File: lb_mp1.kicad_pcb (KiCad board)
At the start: 2 copper layers, 100 x 100 mm, 156 parts, among them J1 USB_POWER, J2 USB_HOST, J3 AudioJack4_SwitchTR1, J4 RJ45_LED_Shielded, J5 Micro_SD_Card, J7 SERIAL, J8 UART_Header, J9 Bat, SW1 SW_SPDT, SW2 SW_SPDT, U1 V3S-split, U10 FPC_40, U11 STM32F030C8Tx, U2 SRV05-4, U3 SY8088AAC, U4 W25Q128JVS, U5 FEMDRM008G-58A39_NO_NC, U6 AMS1117-3.3, U7 CH340N, U8 AXP209, U9 SY7200AABC, Y1 32.768khz, Y2 24MHz

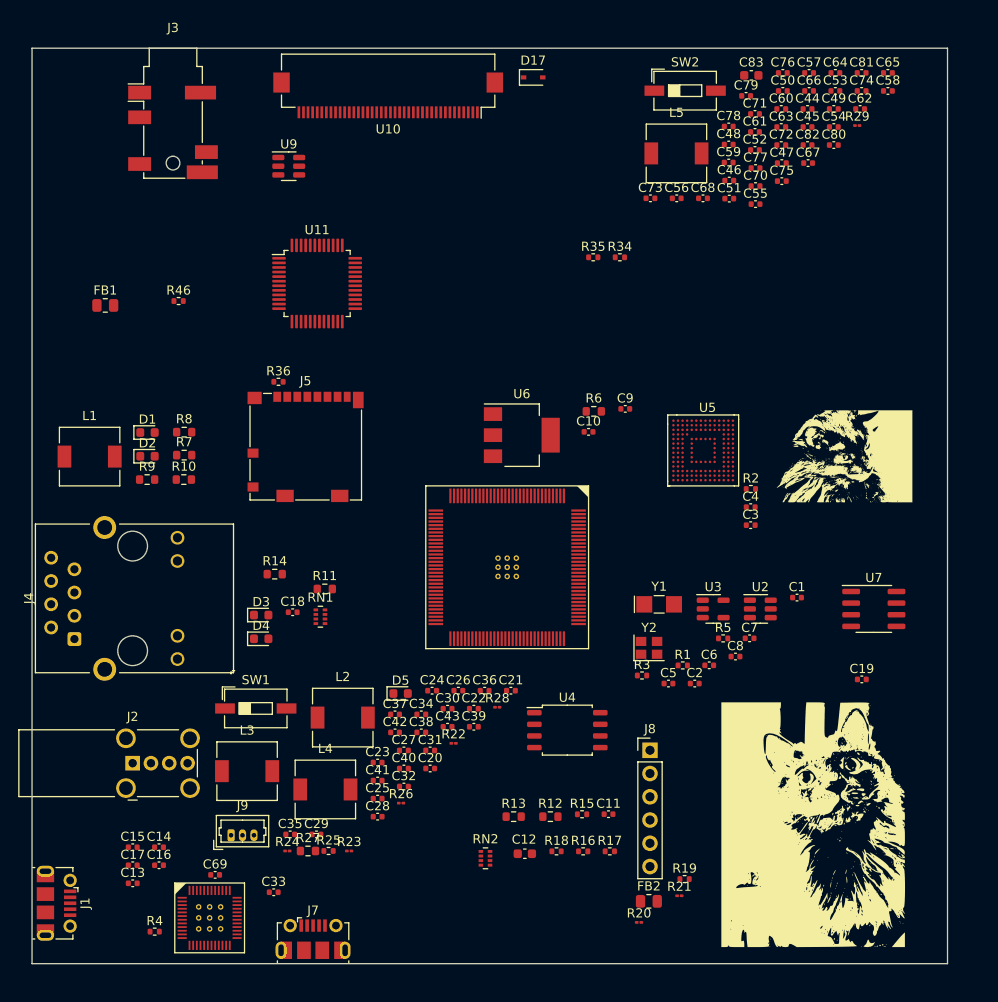
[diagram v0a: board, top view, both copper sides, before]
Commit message: cleaning and naming
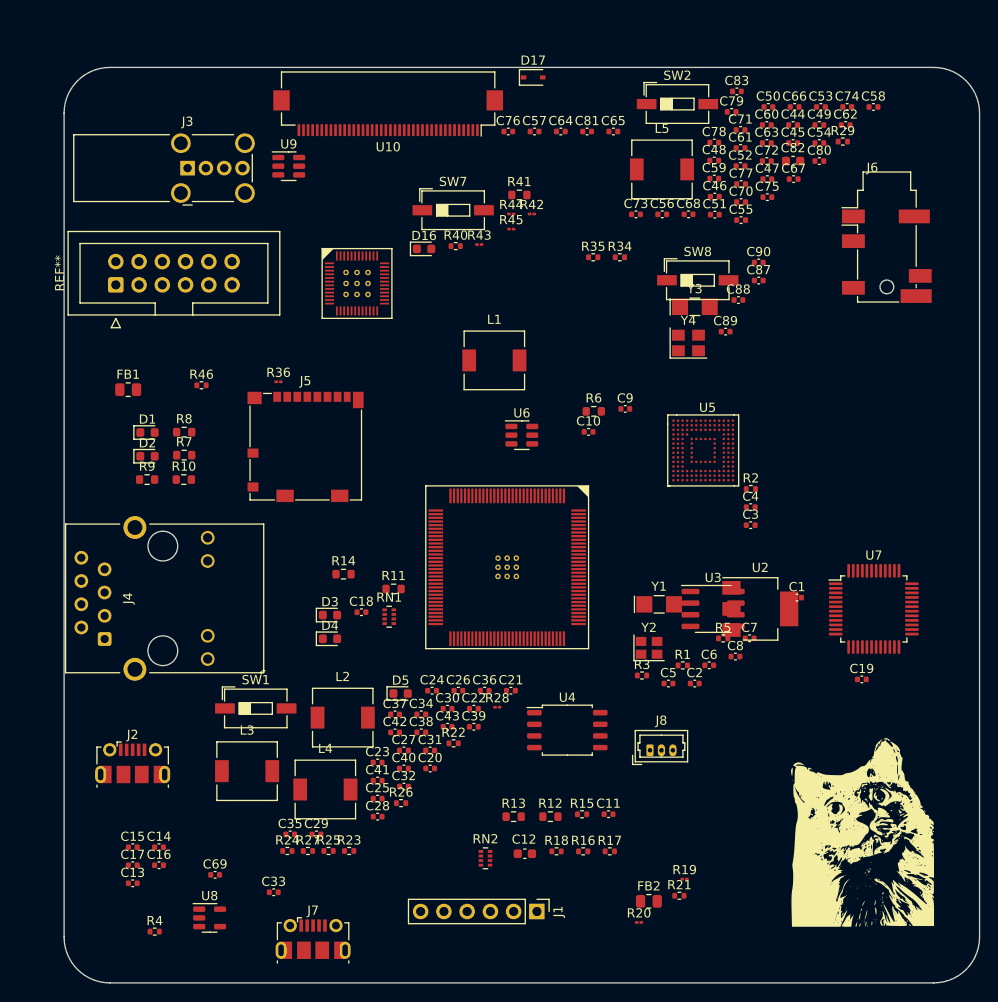
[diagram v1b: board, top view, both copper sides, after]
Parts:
- removed the G*** at (175.2, 72.5)
- removed the G*** at (171.8, 112.7)
- removed J9: Bat, Connector_Molex:Molex_PicoBlade_53047-0310_1x03_P1.25mm_Vertical
- added C87: 12pf, Capacitor_SMD:C_0402_1005Metric, F.Cu at (165.9, 53.3)
- added C88: 12pf, Capacitor_SMD:C_0402_1005Metric, F.Cu at (163.7, 55.4)
- added C89: 18pf, Capacitor_SMD:C_0402_1005Metric, F.Cu at (162.3, 58.9)
- added C90: 18pf, Capacitor_SMD:C_0402_1005Metric, F.Cu at (165.9, 51.3)
- added D16: LED, LED_SMD:LED_0603_1608Metric, F.Cu at (129.3, 49.8)
- added G***: LOGO, LOGO, F.Cu at (175.0, 116.1)
- added J6: AudioJack4_SwitchTR1, Connector_Audio:Jack_3.5mm_PJ31060-I_Horizontal, F.Cu at (179.9, 50.6)
- added R40: 0R, Resistor_SMD:R_0402_1005Metric, F.Cu at (132.8, 49.5)
- added R41: 0.03R, Resistor_SMD:R_0603_1608Metric, F.Cu at (139.7, 43.9)
- added R42: 1k, Resistor_SMD:R_01005_0402Metric, F.Cu at (141.1, 46.0)
- added R43: 200k 1%, Resistor_SMD:R_01005_0402Metric, F.Cu at (135.4, 49.4)
- added R44: 47k, Resistor_SMD:R_01005_0402Metric, F.Cu at (138.8, 46.0)
- added R45: 10k, Resistor_SMD:R_01005_0402Metric, F.Cu at (138.8, 47.7)
- added REF**: IDC-Header_2x06_P2.54mm_Vertical, Connector_IDC:IDC-Header_2x06_P2.54mm_Vertical, F.Cu at (95.7, 53.8)
- added SW7: SW_SPDT, Button_Switch_SMD:SW_DIP_SPSTx01_Slide_6.7x4.1mm_W6.73mm_P2.54mm_LowProfile_JPin, F.Cu at (132.5, 45.6)
- added SW8: SW_SPDT, Button_Switch_SMD:SW_DIP_SPSTx01_Slide_6.7x4.1mm_W6.73mm_P2.54mm_LowProfile_JPin, F.Cu at (159.2, 53.2)
- added Y3: 32.768khz, Crystal:Crystal_SMD_MicroCrystal_CC7V-T1A-2Pin_3.2x1.5mm_HandSoldering, F.Cu at (158.9, 56.1)
- added Y4: 16MHz, Crystal:Crystal_SMD_3225-4Pin_3.2x2.5mm, F.Cu at (158.2, 60.1)
- C11, C19, C67: value 100n -> 10u
- C18: value 0.1uF -> 10u
- C2: value 10u -> 0.1uF
- C22, C27, C41, C42: value 10uF -> 100n
- C23, C25: value 1nF -> 1u
- C24, C26, C39: value 10uF -> 1u
- C28: value 100n -> 1u
- C29, C36: value 1uF -> 100n
- C30: value 4.7uF -> 1u
- C31, C32: value 4.7uF -> 100n
- C33: value 1uF -> 10n
- C34: value 100uF -> 100n
- C35: value 4.7u -> 100n
- C37, C43: value 0.22uF -> 100n
- C38, C44, C46, C48, C50: value 1u -> 100n
- C40: value 10uF -> 10u
- C45: value 1u -> 10u
- C5, C6: value 10u -> 100n
- C52, C56, C61, C63, C65, C66: value 100n -> 10uF
- C54, C60: value 100n -> 4.7uF
- C57, C68, C78: value 100n -> 1uF
- C58: value 1u -> 4.7uF
- C59: value 10u -> 4.7uF
- C62, C64: value 100n -> 1nF
- C69: value 4.7uF -> 100uF
- C70: value 100pF -> 4.7u
- C71: value 10n -> 100pF
- C72: value 10u -> 1uF
- C73: value 100n -> 0.22uF
- C74: value 100pF -> 10uF
- C75: value 10u -> 10uF
- C77: value 100n -> 100pF
- C80: value 1uF -> 4.7uF
- C81: value 4.7uF -> 10uF
- C82: footprint Capacitor_SMD:C_0402_1005Metric -> Capacitor_SMD:C_0603_1608Metric
- C83: value 10uF -> 0.22uF; footprint Capacitor_SMD:C_0603_1608Metric -> Capacitor_SMD:C_0402_1005Metric
- J1: value USB_POWER -> UART_Header; footprint Connector_USB:USB_Micro-B_Molex-105017-0001 -> Connector_PinHeader_2.54mm:PinHeader_1x06_P2.54mm_Vertical
- J2: value USB_HOST -> SERIAL; footprint Connector_USB:USB_A_Wuerth_614004134726_Horizontal -> Connector_USB:USB_Micro-B_Molex-105017-0001
- J3: value AudioJack4_SwitchTR1 -> USB_HOST; footprint Connector_Audio:Jack_3.5mm_PJ31060-I_Horizontal -> Connector_USB:USB_A_Wuerth_614004134726_Horizontal
- J7: value SERIAL -> USB_POWER
- J8: value UART_Header -> Bat; footprint Connector_PinHeader_2.54mm:PinHeader_1x06_P2.54mm_Vertical -> Connector_Molex:Molex_PicoBlade_53047-0310_1x03_P1.25mm_Vertical
- R19: value 47k -> 470; footprint Resistor_SMD:R_0402_1005Metric -> Resistor_SMD:R_01005_0402Metric
- R21: value 470 -> 47k; footprint Resistor_SMD:R_01005_0402Metric -> Resistor_SMD:R_0402_1005Metric
- R22: value 2.2R -> 33R; footprint Resistor_SMD:R_01005_0402Metric -> Resistor_SMD:R_0402_1005Metric
- R23: value 1k -> 10k; footprint Resistor_SMD:R_01005_0402Metric -> Resistor_SMD:R_0402_1005Metric
- R24: value 47k -> 33R; footprint Resistor_SMD:R_01005_0402Metric -> Resistor_SMD:R_0402_1005Metric
- R25: value 47k -> 33R
- R26: value 200k 1% -> 0R; footprint Resistor_SMD:R_01005_0402Metric -> Resistor_SMD:R_0402_1005Metric
- R27: value 0.03R -> 22R; footprint Resistor_SMD:R_0603_1608Metric -> Resistor_SMD:R_0402_1005Metric
- R29: value 1k -> 47k; footprint Resistor_SMD:R_01005_0402Metric -> Resistor_SMD:R_0402_1005Metric
- R36: value 33R -> 1k; footprint Resistor_SMD:R_0402_1005Metric -> Resistor_SMD:R_01005_0402Metric
- R46: value 0R -> 10k
- U11: value STM32F030C8Tx -> AXP209; footprint Package_QFP:LQFP-48_7x7mm_P0.5mm -> Allwinner:AXP209-QFN48
- U2: value SRV05-4 -> AMS1117-3.3; footprint Package_TO_SOT_SMD:SOT-23-6 -> Package_TO_SOT_SMD:SOT-223-3_TabPin2
- U3: value SY8088AAC -> CH340N; footprint Package_TO_SOT_SMD:SOT-23-5 -> Package_SO:SOIC-8_3.9x4.9mm_P1.27mm
- U6: value AMS1117-3.3 -> SRV05-4; footprint Package_TO_SOT_SMD:SOT-223-3_TabPin2 -> Package_TO_SOT_SMD:SOT-23-6
- U7: value CH340N -> STM32F030C8Tx; footprint Package_SO:SOIC-8_3.9x4.9mm_P1.27mm -> Package_QFP:LQFP-48_7x7mm_P0.5mm
- U8: value AXP209 -> SY8088AAC; footprint Allwinner:AXP209-QFN48 -> Package_TO_SOT_SMD:SOT-23-5
- moved J1 52.5 mm to (141.7, 122.2)
- moved L1 45.4 mm to (137.0, 62.0)
- moved C57 30.7 mm to (141.4, 37.0)
- moved C64 30.7 mm to (144.3, 37.0)
- moved C65 30.7 mm to (150.0, 37.0)
- moved C81 30.7 mm to (147.1, 37.0)
- moved C76 30.7 mm to (138.5, 37.0)
- moved FB1 9.53 mm to (97.0, 65.2)
- moved R46 9.53 mm to (105.0, 64.7)
- moved C18 7.51 mm to (122.5, 89.5)
- moved D3 7.51 mm to (119.0, 89.8)
- moved D4 7.51 mm to (119.0, 92.4)
- moved R11 7.51 mm to (126.0, 87.0)
- moved RN1 7.51 mm to (125.5, 90.0)
- moved R14 7.51 mm to (120.5, 85.3)
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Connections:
- C1 pad 2: Net-(C1-Pad2) -> GND
- C11 pad 1: +3.3V -> +1V2
- C18 pad 1: Net-(C18-Pad1) -> +1V2
- C19 pad 1: Net-(C19-Pad1) -> +3.3V
- C2 pad 1: +1V2 -> Net-(C2-Pad1)
- C22 pad 1: +1V2 -> +3.3V
- C24 pad 1: +3.3V -> +1V2
- C26 pad 1: +3.3V -> +1V8
- C29 pad 1: GND -> +1V2
- C29 pad 2: VDD -> GND
- C30 pad 1: GND -> +1V2
- C30 pad 2: +3V0 -> GND
- C31 pad 1: GND -> +3.3V
- C31 pad 2: Net-(C31-Pad2) -> GND
- C32 pad 1: Net-(C32-Pad1) -> +1V8
- C33 pad 1: GND -> +VDC
- C33 pad 2: Net-(C33-Pad2) -> GND
- C34 pad 1: GND -> VDD
- C34 pad 2: Net-(C34-Pad2) -> GND
- C35 pad 1: GND -> +3V0
- C35 pad 2: Net-(C35-Pad2) -> GND
- C36 pad 1: Net-(C36-Pad1) -> +1V2
- C37 pad 1: VCC -> +1V2
- C38 pad 1: +1V2 -> +3.3V
- C39 pad 1: VCC -> +1V8
- C40 pad 1: VCC -> +3V0
- C41 pad 1: VCC -> +1V2
- C42 pad 1: Net-(C42-Pad1) -> +1V2
- C43 pad 1: VCC -> +1V8
- C44 pad 1: +1V2 -> +3.3V
- C45 pad 1: +3.3V -> +VDC
- C46 pad 1: +1V8 -> +1V2
- C47 pad 1: +3.3V -> +1V2
- C48 pad 1: +3.3V -> +3V0
- C49 pad 1: +1V2 -> +VDC
- C5 pad 1: +1V2 -> +3.3V
- C50 pad 1: +1V2 -> +1V8
- C50 pad 2: GND -> Net-(C50-Pad2)
- C51 pad 1: +3.3V -> Net-(C50-Pad2)
- C52 pad 1: +1V8 -> VCC
- C53 pad 1: VDD -> +1V8
- C53 pad 2: GND -> Net-(C53-Pad2)
- C54 pad 1: +3V0 -> GND
- C54 pad 2: GND -> Net-(C54-Pad2)
- C55 pad 1: +1V2 -> +1V8
- C56 pad 1: +1V2 -> +1V8
- C57 pad 1: +3.3V -> GND
- C57 pad 2: GND -> VDD
- C58 pad 1: +1V8 -> GND
- C58 pad 2: GND -> +3V0
- C59 pad 1: +3V0 -> GND
- C59 pad 2: GND -> Net-(C59-Pad2)
- C6 pad 1: +3.3V -> Net-(C6-Pad1)
- C6 pad 2: GND -> Net-(C6-Pad2)
- C60 pad 1: +1V2 -> Net-(C60-Pad1)
- C62 pad 1: +1V8 -> +1V2
- C64 pad 1: +1V2 -> +3.3V
- C65 pad 1: +1V2 -> +3.3V
- C66 pad 1: +3V0 -> +3.3V
- C67 pad 1: +1V8 -> GND
- C67 pad 2: Net-(C67-Pad2) -> +VDC
- C68 pad 1: Net-(C67-Pad2) -> GND
- C68 pad 2: GND -> Net-(C68-Pad2)
- C70 pad 2: N_Oe -> Net-(C70-Pad2)
- C71 pad 1: +VDC -> GND
- C71 pad 2: GND -> N_Oe
- C72 pad 1: +VDC -> Net-(C72-Pad1)
- C73 pad 1: +VDC -> VCC
- C74 pad 1: GND -> VCC
- C74 pad 2: Pwron -> GND
- C75 pad 1: GND -> VCC
- C75 pad 2: +VDC -> GND
- C77 pad 1: +1V8 -> GND
- C77 pad 2: Net-(C77-Pad2) -> Pwron
- C78 pad 1: +1V8 -> +BATT
- C78 pad 2: GND -> Net-(C78-Pad2)
- C79 pad 1: +1V8 -> Net-(C78-Pad2)
- C80 pad 1: +BATT -> Net-(C80-Pad1)
- C80 pad 2: Net-(C42-Pad1) -> GND
- C81 pad 1: Net-(C81-Pad1) -> +BATT
- C82 pad 1: +BATT -> VCC
- FB1 pad 1: Net-(U11-Pad9) -> Net-(FB1-Pad1)
- FB1 pad 2: +3.3V -> Net-(C2-Pad1)
- FB2 pad 2: Net-(C18-Pad1) -> +3.3V
- J1 pad 1: +VDC -> GND
- J1 pad 4: Net-(J1-Pad4) -> Net-(D4-Pad1)
- J1 pad 5: GND -> Net-(D5-Pad1)
- J1 pad 6: GND -> unconnected-(J1-Pad6)
- J2 pad 1: VCC -> Net-(FB1-Pad1)
- J2 pad 4: GND -> Net-(J2-Pad4)
- J5 pad 1: Net-(D11-Pad1) -> Net-(D7-Pad1)
- J5 pad 2: Net-(D12-Pad1) -> Net-(D8-Pad1)
- J5 pad 5: Net-(D10-Pad1) (its old number) -> Net-(D6-Pad1)
- J5 pad 8: Net-(D15-Pad1) -> Net-(D11-Pad1)
- J7 pad 1: Net-(FB2-Pad1) -> +VDC
- J7 pad 2: Net-(J7-Pad2) -> unconnected-(J7-Pad2)
- J7 pad 3: Net-(J7-Pad3) -> unconnected-(J7-Pad3)
- J8 pad 1: GND -> +BATT
- J8 pad 2: unconnected-(J8-Pad2) -> GND
- J8 pad 3: unconnected-(J8-Pad3) -> (no net)
- L2 pad 1: +1V2 -> Net-(L2-Pad1)
- L2 pad 2: Net-(L2-Pad2) -> +1V8
- L3 pad 1: +3.3V -> +1V2
- L4 pad 1: Net-(L4-Pad1) -> +3.3V
- L4 pad 2: Net-(C42-Pad1) -> Net-(L4-Pad2)
- L5 pad 2: +1V8 -> Net-(C78-Pad2)
- R19 pad 1: Net-(J7-Pad4) -> +3.3V
- R19 pad 2: GND -> Net-(D4-Pad2)
- R20 pad 2: Net-(D3-Pad2) -> Net-(D5-Pad2)
- R21 pad 1: +3.3V -> Net-(J2-Pad4)
- R21 pad 2: Net-(D4-Pad2) -> GND
- R22 pad 1: +5V -> Net-(D6-Pad1)
- R22 pad 2: Net-(C20-Pad1) -> Net-(R22-Pad2)
- R23 pad 1: GND -> +3.3V
- R23 pad 2: N_Oe -> Net-(D7-Pad1)
- R24 pad 1: reset -> Net-(D14-Pad1)
- R24 pad 2: VDD -> Net-(R24-Pad2)
- R25 pad 1: Net-(J1-Pad4) -> Net-(D13-Pad1)
- R25 pad 2: GND -> Net-(R25-Pad2)
- R26 pad 1: GND -> Net-(C6-Pad2)
- R27 pad 1: Net-(C42-Pad1) -> GND
- R27 pad 2: +BATT -> Net-(C6-Pad1)
- R29 pad 1: Net-(R29-Pad1) -> Net-(J7-Pad4)
- R29 pad 2: Pwron -> GND
- R36 pad 1: Net-(D10-Pad1) (its old number) -> GND
- R36 pad 2: Net-(R36-Pad2) -> N_Oe
- R46 pad 1: VCC -> +3.3V
- R46 pad 2: Net-(C81-Pad1) -> Net-(U4-Pad3)
- RN1 pad 2: Net-(D12-Pad1) -> Net-(D8-Pad1)
- RN1 pad 5: Net-(D15-Pad1) -> Net-(D11-Pad1)
- U1 pad 101: Net-(D11-Pad1) -> Net-(D7-Pad1)
- U1 pad 102: Net-(D12-Pad1) -> Net-(D8-Pad1)
- U1 pad 105: Net-(R36-Pad2) -> Net-(R22-Pad2)
- U1 pad 107: Net-(D15-Pad1) -> Net-(D11-Pad1)
- U1 pad 110: Net-(J2-Pad2) -> Net-(J3-Pad2)
- U1 pad 111: Net-(J2-Pad3) -> Net-(J3-Pad3)
- U1 pad 120: Net-(R34-Pad2) -> Net-(R25-Pad2)
- U1 pad 121: Net-(R35-Pad2) -> Net-(R24-Pad2)
- U1 pad 124: Net-(C1-Pad2) -> Net-(C6-Pad2)
- U1 pad 125: Net-(R1-Pad2) -> Net-(R26-Pad2)
- U1 pad 48: Net-(D3-Pad1) -> Net-(D5-Pad1)
- U1 pad 63: Net-(C67-Pad2) -> Net-(C50-Pad2)
- U1 pad 71: Net-(C67-Pad2) -> Net-(C50-Pad2)
- U1 pad 73: Net-(R22-Pad2) -> Net-(R35-Pad2)
- U1 pad 97: Net-(C69-Pad2) -> Net-(C54-Pad2)
- U11 pad 1: +3.3V -> sda
- U11 pad 10: unconnected-(U11-Pad10) -> +1V2
- U11 pad 11: unconnected-(U11-Pad11) -> Net-(C60-Pad1)
- U11 pad 12: USART1_TX -> +3V0
- U11 pad 13: USART1_RX -> +3.3V
- U11 pad 14: unconnected-(U11-Pad14) -> VCC
- U11 pad 15: unconnected-(U11-Pad15) -> Net-(L4-Pad2)
- U11 pad 16: unconnected-(U11-Pad16) -> GND
- U11 pad 17: unconnected-(U11-Pad17) -> +3.3V
- U11 pad 19: unconnected-(U11-Pad19) -> Net-(C70-Pad2)
- U11 pad 2: unconnected-(U11-Pad2) -> scl
- U11 pad 21: unconnected-(U11-Pad21) -> VCC
- U11 pad 22: unconnected-(U11-Pad22) -> GND
- U11 pad 23: GND -> Net-(R43-Pad2)
- U11 pad 24: +3.3V -> Net-(C68-Pad2)
- U11 pad 25: unconnected-(U11-Pad25) -> reset
- U11 pad 26: unconnected-(U11-Pad26) -> Net-(C72-Pad1)
- U11 pad 27: unconnected-(U11-Pad27) -> Net-(C72-Pad1)
- U11 pad 28: unconnected-(U11-Pad28) -> VDD
- U11 pad 29: unconnected-(U11-Pad29) -> VCC
- U11 pad 30: unconnected-(U11-Pad30) -> Net-(C69-Pad2)
- U11 pad 31: unconnected-(U11-Pad31) -> Net-(C80-Pad1)
- U11 pad 32: unconnected-(U11-Pad32) -> +VDC
- U11 pad 33: unconnected-(U11-Pad33) -> +VDC
- U11 pad 34: unconnected-(U11-Pad34) -> VCC
- U11 pad 35: unconnected-(U11-Pad35) -> VCC
- U11 pad 36: unconnected-(U11-Pad36) -> Net-(D16-Pad1)
- U11 pad 37: unconnected-(U11-Pad37) -> GND
- U11 pad 38: unconnected-(U11-Pad38) -> +BATT
- U11 pad 39: unconnected-(U11-Pad39) -> +BATT
- U11 pad 4: unconnected-(U11-Pad4) -> N_Oe
- U11 pad 40: unconnected-(U11-Pad40) -> +3.3V
- U11 pad 41: unconnected-(U11-Pad41) -> Net-(C59-Pad2)
- U11 pad 42: unconnected-(U11-Pad42) -> +BATT
- U11 pad 43: unconnected-(U11-Pad43) -> Net-(C78-Pad2)
- U11 pad 44: unconnected-(U11-Pad44) -> VCC
- U11 pad 45: unconnected-(U11-Pad45) -> Net-(L5-Pad1)
- U11 pad 46: unconnected-(U11-Pad46) -> GND
- U11 pad 47: GND -> Pwron
- U11 pad 48: +3.3V -> NMI
- U11 pad 6: unconnected-(U11-Pad6) -> GND
- U11 pad 7: Net-(U11-Pad7) -> VCC
- U11 pad 8: GND -> Net-(L3-Pad2)
- U11 pad 9: Net-(U11-Pad9) -> GND
- U2 pad 1: Net-(J2-Pad3) -> GND
- U2 pad 2: GND -> Net-(C1-Pad1)
- U2 pad 3: Net-(J2-Pad2) -> Net-(C2-Pad1)
- U3 pad 1: Net-(R30-Pad2) -> Net-(J2-Pad3)
- U3 pad 2: GND -> Net-(J2-Pad2)
- U3 pad 3: Net-(L5-Pad1) -> GND
- U3 pad 4: VCC -> unconnected-(U3-Pad4)
- U3 pad 5: Net-(C77-Pad2) -> Net-(C2-Pad1)
- U4 pad 3: +3.3V -> Net-(U4-Pad3)
- U4 pad 7: +3.3V -> Net-(U4-Pad3)
- U6 pad 1: GND -> Net-(J3-Pad3)
- U6 pad 2: Net-(C19-Pad1) -> GND
- U6 pad 3: Net-(C18-Pad1) -> Net-(J3-Pad2)
- U7 pad 1: Net-(J7-Pad3) -> +3.3V
- U7 pad 2: Net-(J7-Pad2) -> unconnected-(U7-Pad2)
- U7 pad 3: GND -> OSC32_IN
- U7 pad 4: unconnected-(U7-Pad4) -> OSC32_OUT
- U7 pad 5: Net-(C18-Pad1) -> OSC_IN
- U7 pad 6: Net-(D4-Pad1) -> OSC_OUT
- U7 pad 7: Net-(D3-Pad1) -> Net-(R28-Pad1)
- U7 pad 8: Net-(C19-Pad1) -> GND
- U8 pad 1: sda -> Net-(R32-Pad2)
- U8 pad 2: scl -> GND
- U8 pad 3: unconnected-(U8-Pad3) -> Net-(L2-Pad1)
- U8 pad 4: N_Oe -> VCC
- U8 pad 5: unconnected-(U8-Pad5) -> Net-(C53-Pad2)
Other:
- outline, holes or cut-outs redrawn
